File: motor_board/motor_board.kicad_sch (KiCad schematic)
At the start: 0 parts

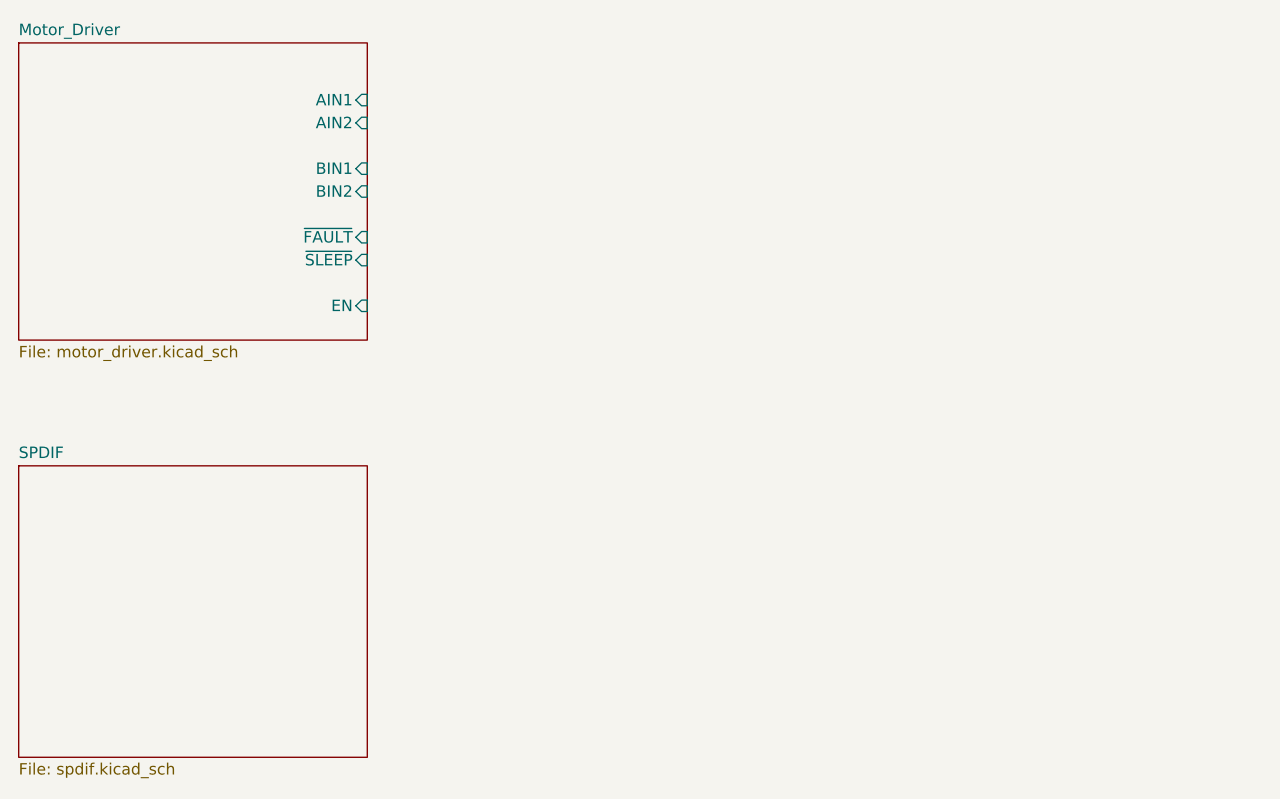
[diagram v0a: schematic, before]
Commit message: Began motor board layour
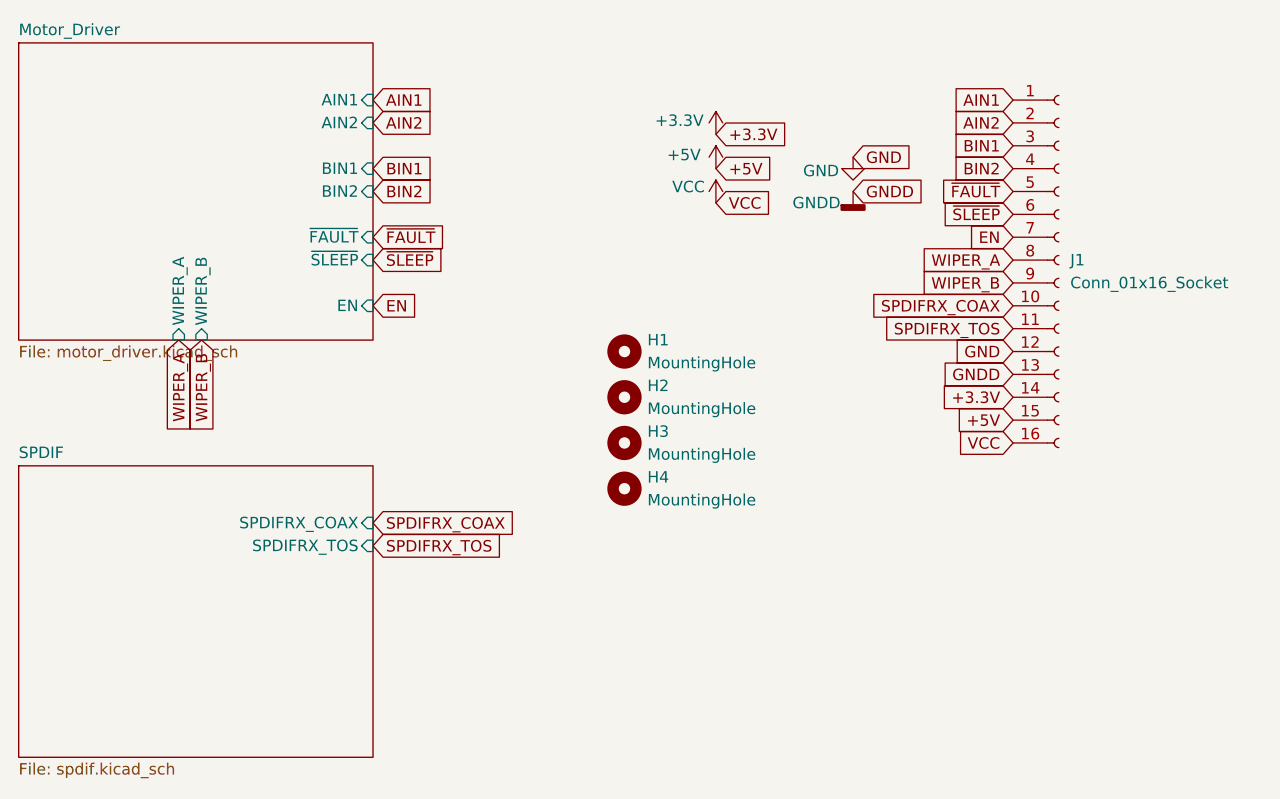
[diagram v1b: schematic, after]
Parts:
- added H1, H2, H3, H4: MountingHole, MountingHole:MountingHole_3.2mm_M3, symbol Mechanical:MountingHole
- added J1: Conn_01x16_Socket, Connector_JST:JST_PH_S16B-PH-K_1x16_P2.00mm_Horizontal, symbol Connector:Conn_01x16_Socket
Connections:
- new net +3.3V: J1.14 (Pin_14)
- new net +5V: J1.15 (Pin_15)
- new net AIN1: J1.1 (Pin_1)
- new net AIN2: J1.2 (Pin_2)
- new net BIN1: J1.3 (Pin_3)
- new net BIN2: J1.4 (Pin_4)
- new net EN: J1.7 (Pin_7)
- new net GND: J1.12 (Pin_12)
- new net GNDD: J1.13 (Pin_13)
- new net SPDIFRX_COAX: J1.10 (Pin_10)
- new net SPDIFRX_TOS: J1.11 (Pin_11)
- new net VCC: J1.16 (Pin_16)
- new net WIPER_A: J1.8 (Pin_8)
- new net WIPER_B: J1.9 (Pin_9)
- new net ~{FAULT}: J1.5 (Pin_5)
- new net ~{SLEEP}: J1.6 (Pin_6)
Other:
- sheet Motor_Driver ports: added WIPER_A, WIPER_B; removed none
- sheet SPDIF ports: added SPDIFRX_COAX, SPDIFRX_TOS; removed none
